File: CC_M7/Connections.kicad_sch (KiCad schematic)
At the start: 11 parts, among them J1 Conn_01x04_Pin, J10 Conn_01x04_Pin, J11 USB_B_Micro, J12 Conn_01x04_Pin, J3 Conn_01x03_Pin, J4 Conn_01x03_Pin, J5 Conn_01x03_Pin, J6 Conn_01x03_Pin, J7 Conn_01x03_Pin, J8 Conn_01x03_Pin

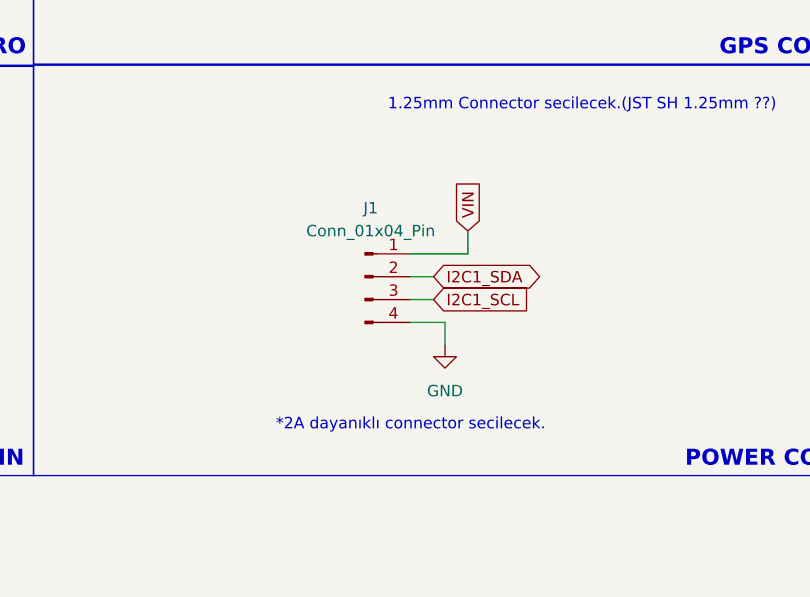
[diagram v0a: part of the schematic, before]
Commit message: ready to start PCB drawing
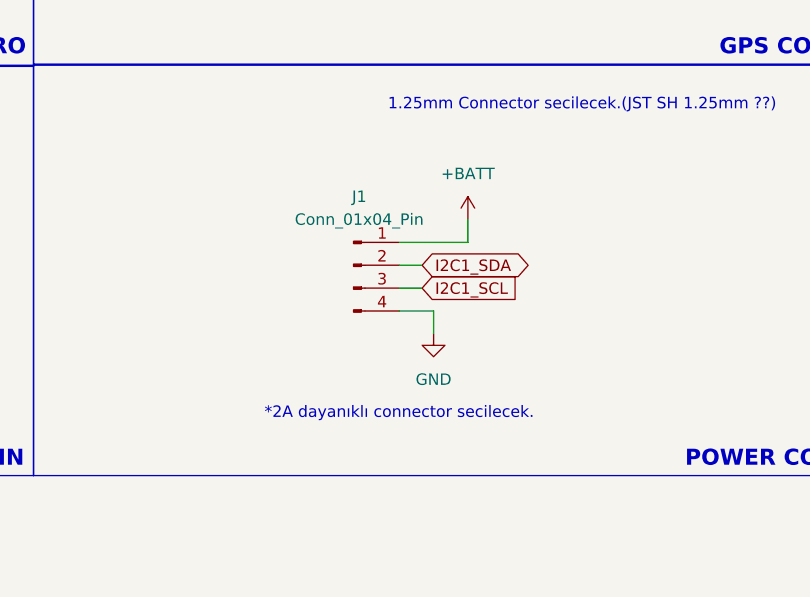
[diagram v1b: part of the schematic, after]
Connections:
- net VIN renamed +BATT
